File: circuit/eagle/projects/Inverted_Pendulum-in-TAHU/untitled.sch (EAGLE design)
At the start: 16 parts, among them X3 332-02

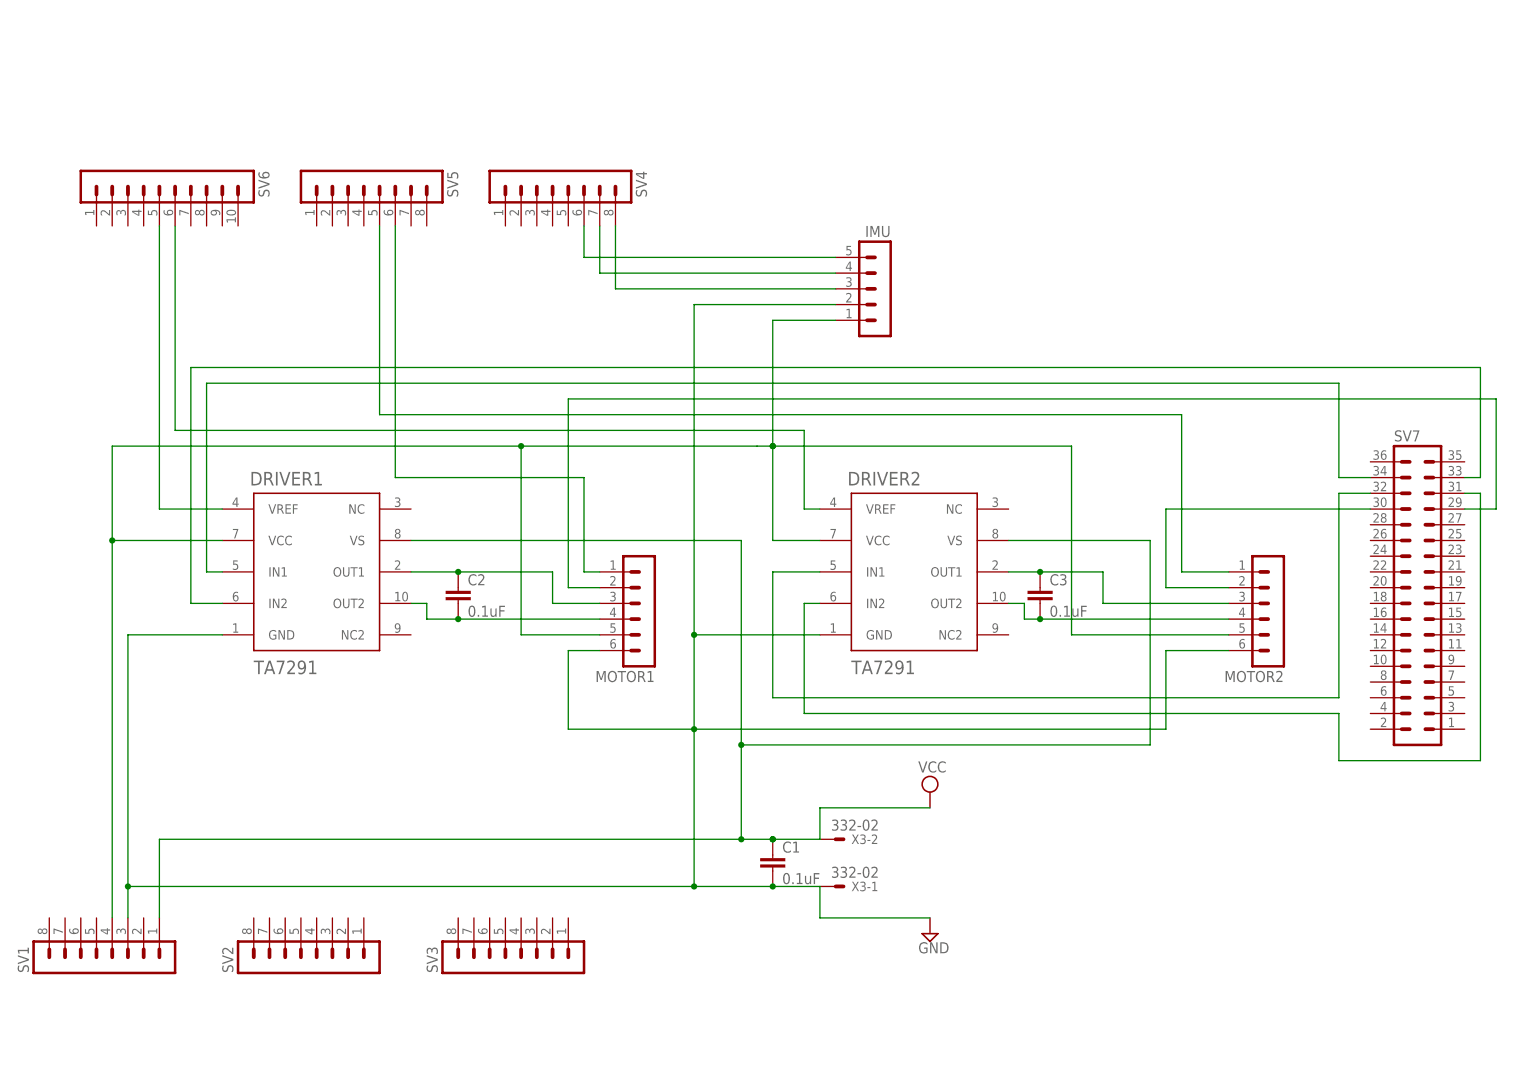
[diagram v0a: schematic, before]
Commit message: Update circuit
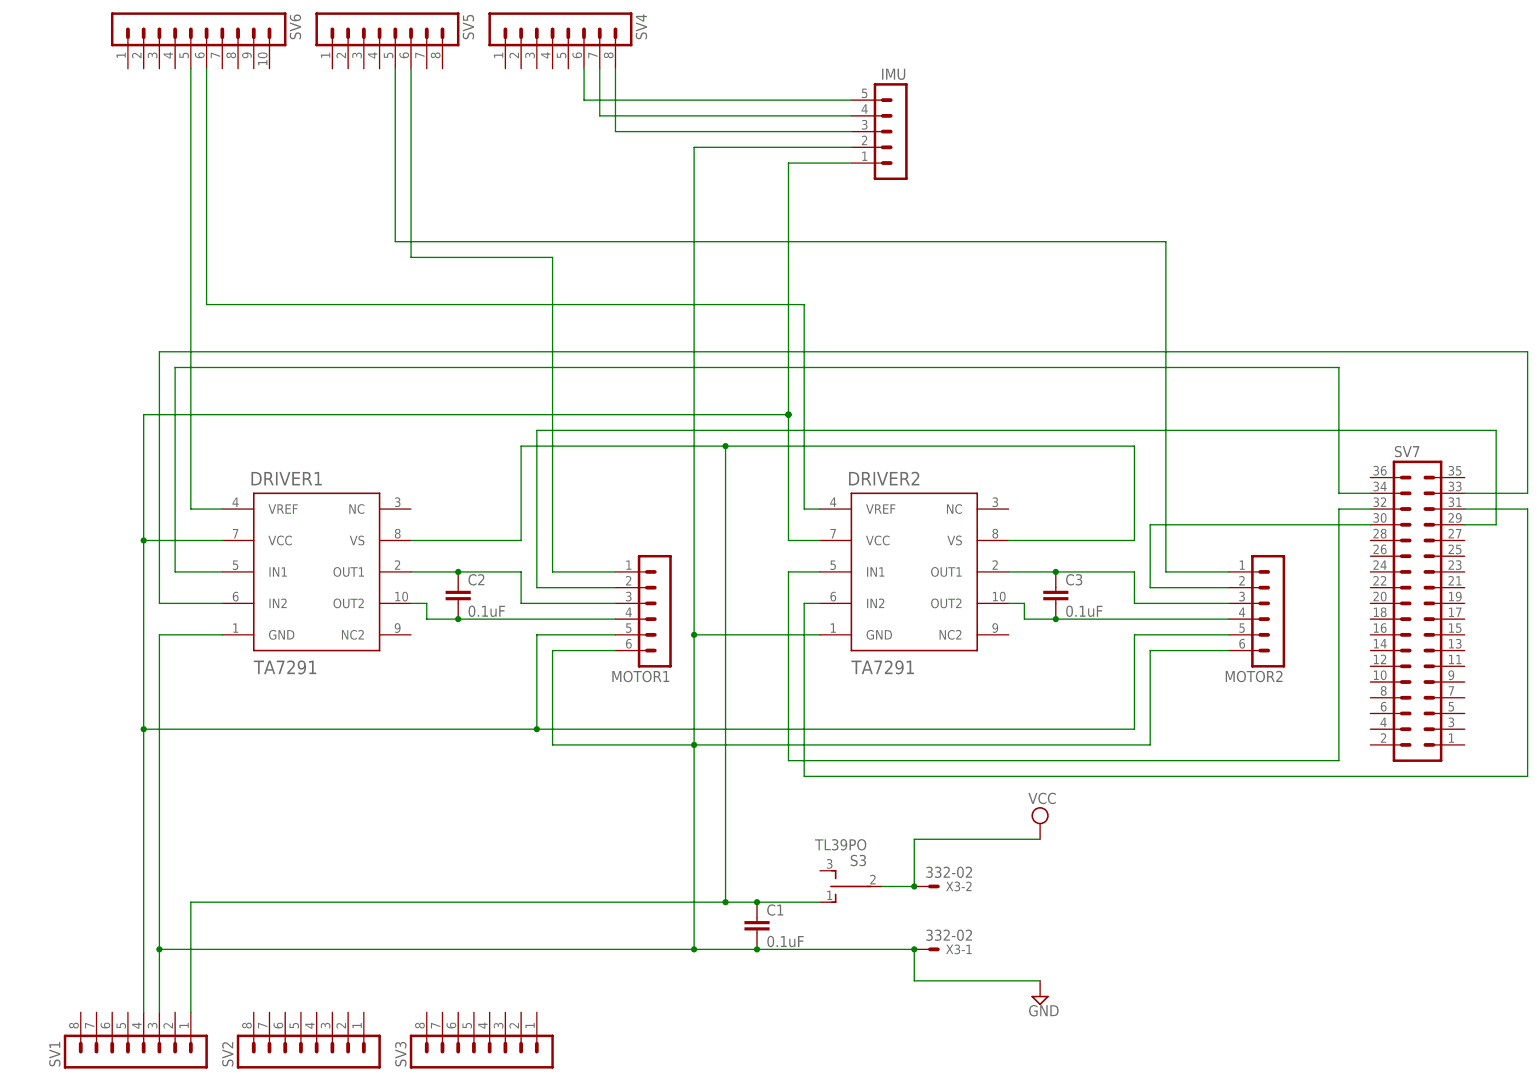
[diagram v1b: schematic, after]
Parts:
- added S3: TL39PO, switch:TL39PO
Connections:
- net N$10: now also C1.1, DRIVER1.VS, DRIVER2.VS, S3.O, SV1.1; no longer DRIVER1.VCC, MOTOR1.5, SV1.4
- net N$7: now also DRIVER1.VCC, MOTOR1.5, SV1.4
- net VCC: now also S3.P; no longer C1.1, DRIVER1.VS, DRIVER2.VS, SV1.1
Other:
- moved on the sheet: C1, C3, IMU, MOTOR1, SV1, SV2, SV3, SV4, SV5, SV6, SV7, X3-1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
